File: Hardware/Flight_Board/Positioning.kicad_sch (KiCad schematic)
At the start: 24 parts, among them J5 GPS_ANT, J6 EXT_GPS, Q2 NMOS, SW4 DPDT_Slide_SMD, U4 BMP390, U5 NEO-M8N

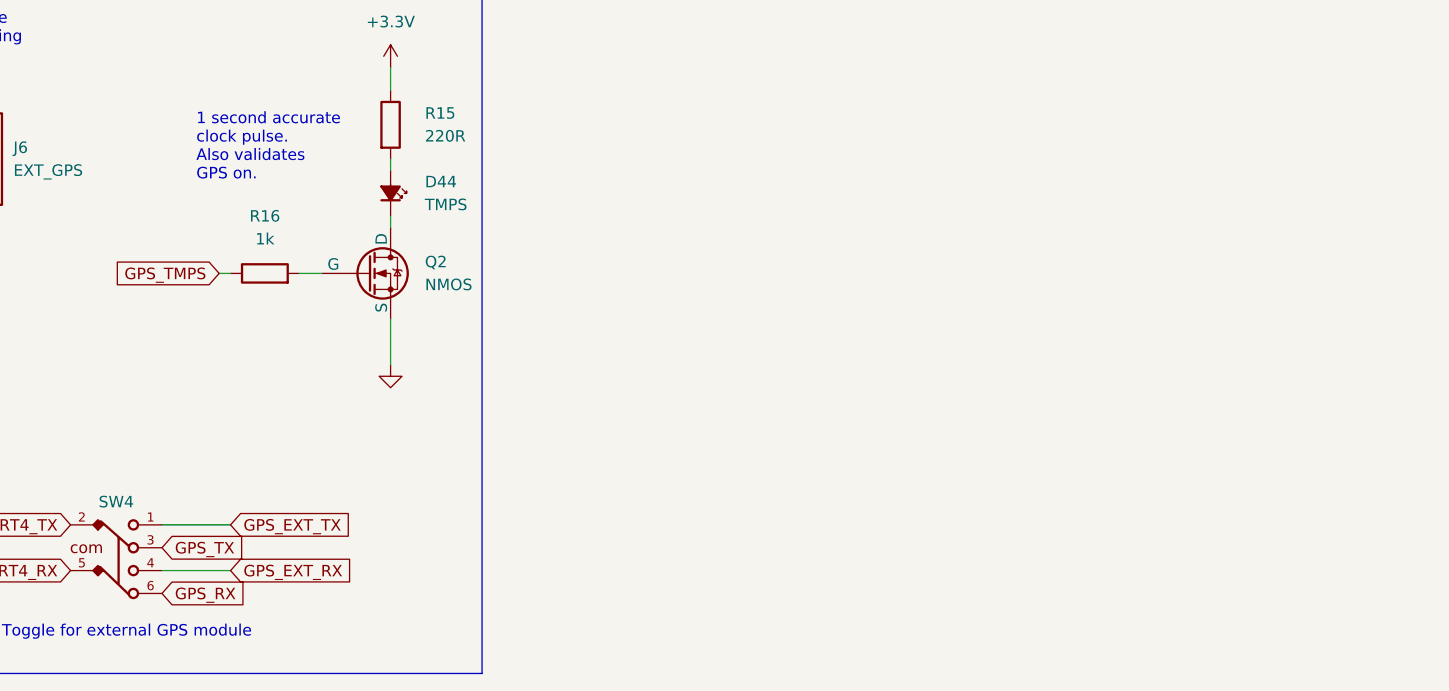
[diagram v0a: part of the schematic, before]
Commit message: ESC Rough Draft
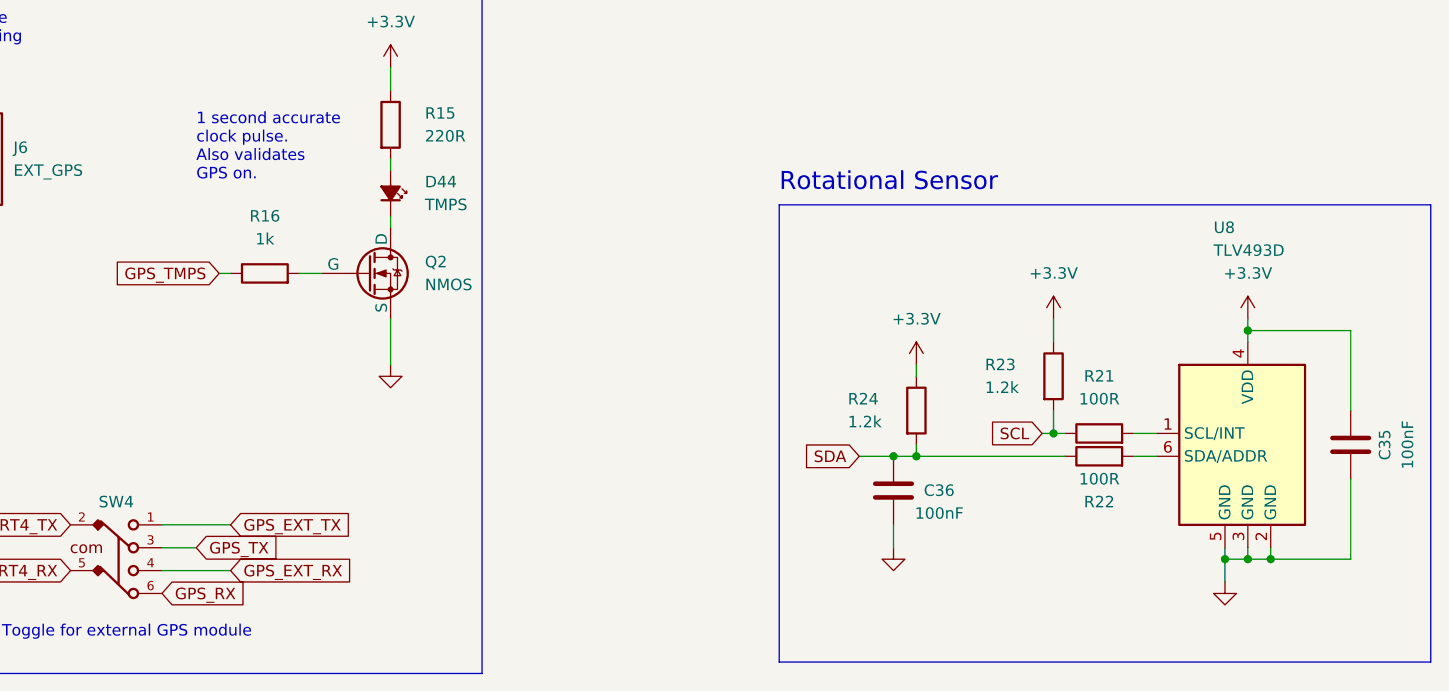
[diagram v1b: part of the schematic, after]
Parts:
- added C35, C36: 100nF, symbol Device:C
- added R21, R22: 100R, symbol Device:R
- added R23, R24: 1.2k, symbol Device:R
- added U8: TLV493D, Package_TO_SOT_SMD:SOT-23-6, symbol Sensor_Magnetic:TLV493D
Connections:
- net +3.3V: now also C35.2, R23.1, R24.1, U8.4 (VDD)
- net GND: now also C35.1, C36.1, U8.2 (GND), U8.3 (GND), U8.5 (GND)
- new net: R21.2, U8.1 (SCL/INT)
- new net: R22.2, U8.6 (SDA/ADDR)
- new net SCL: R21.1, R23.2
- new net SDA: C36.2, R22.1, R24.2
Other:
- note added: "Rotational Sensor"
